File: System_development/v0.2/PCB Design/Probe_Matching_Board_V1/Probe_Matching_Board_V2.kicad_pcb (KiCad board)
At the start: 2 copper layers, 10.4 x 40.8 mm, 4 parts, among them J1 Conn_Coaxial, J2 Conn_Coaxial

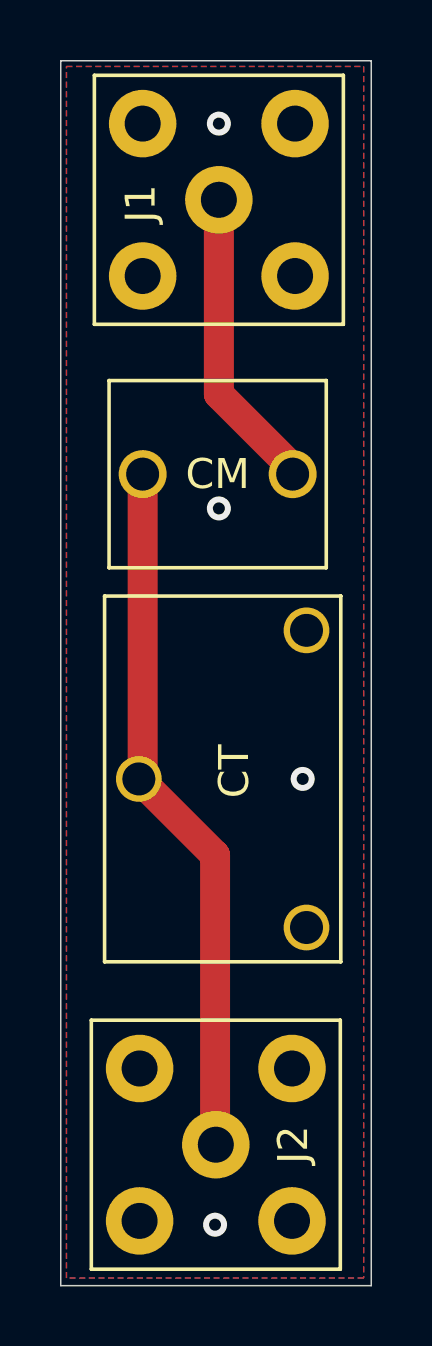
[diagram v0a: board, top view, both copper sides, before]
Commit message: New tray design and File organization
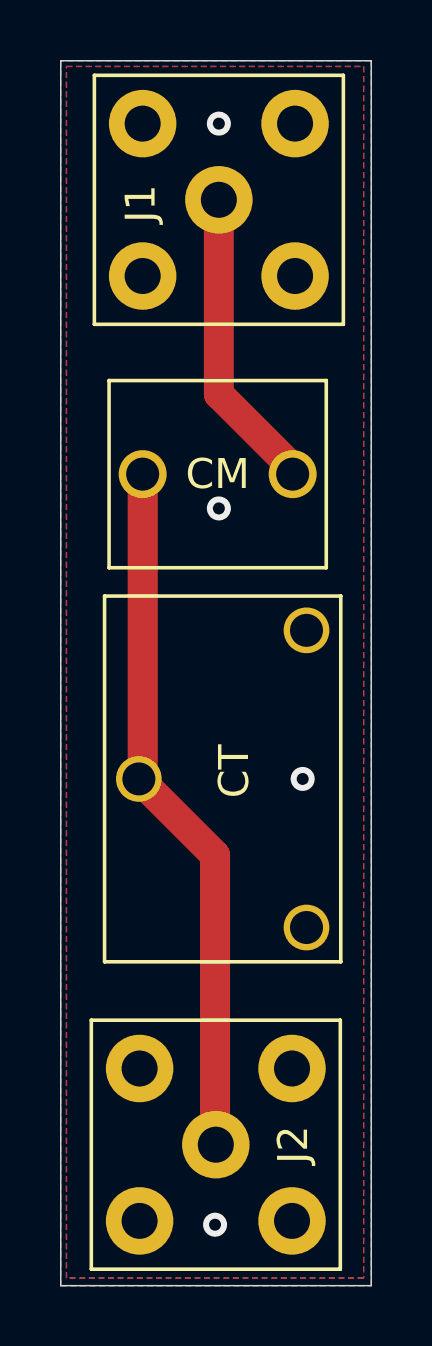
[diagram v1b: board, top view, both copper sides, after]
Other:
- net class Default removed
